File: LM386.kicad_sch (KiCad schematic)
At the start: 16 parts, among them J1 Conn_01x02_Pin, J2 Conn_01x02_Pin, U1 LM386, U2 LM386

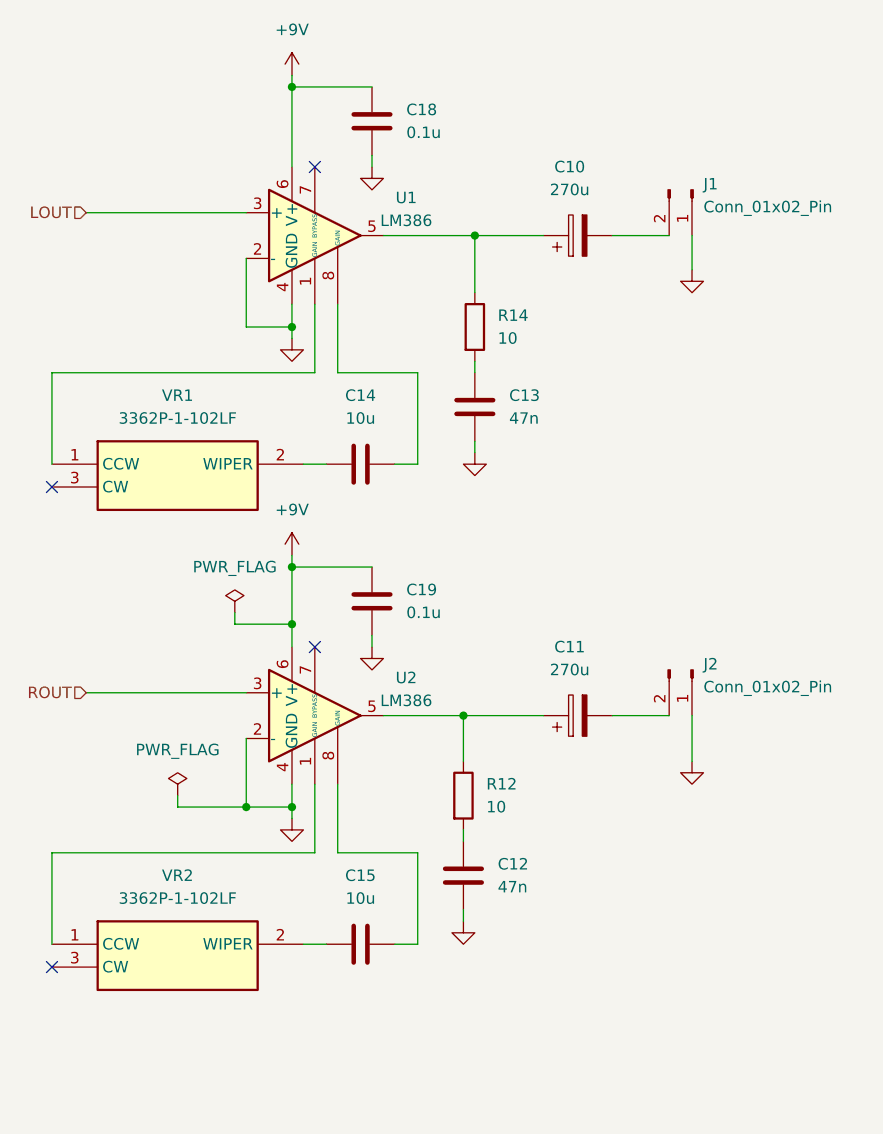
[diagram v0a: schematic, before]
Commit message: Complete layout
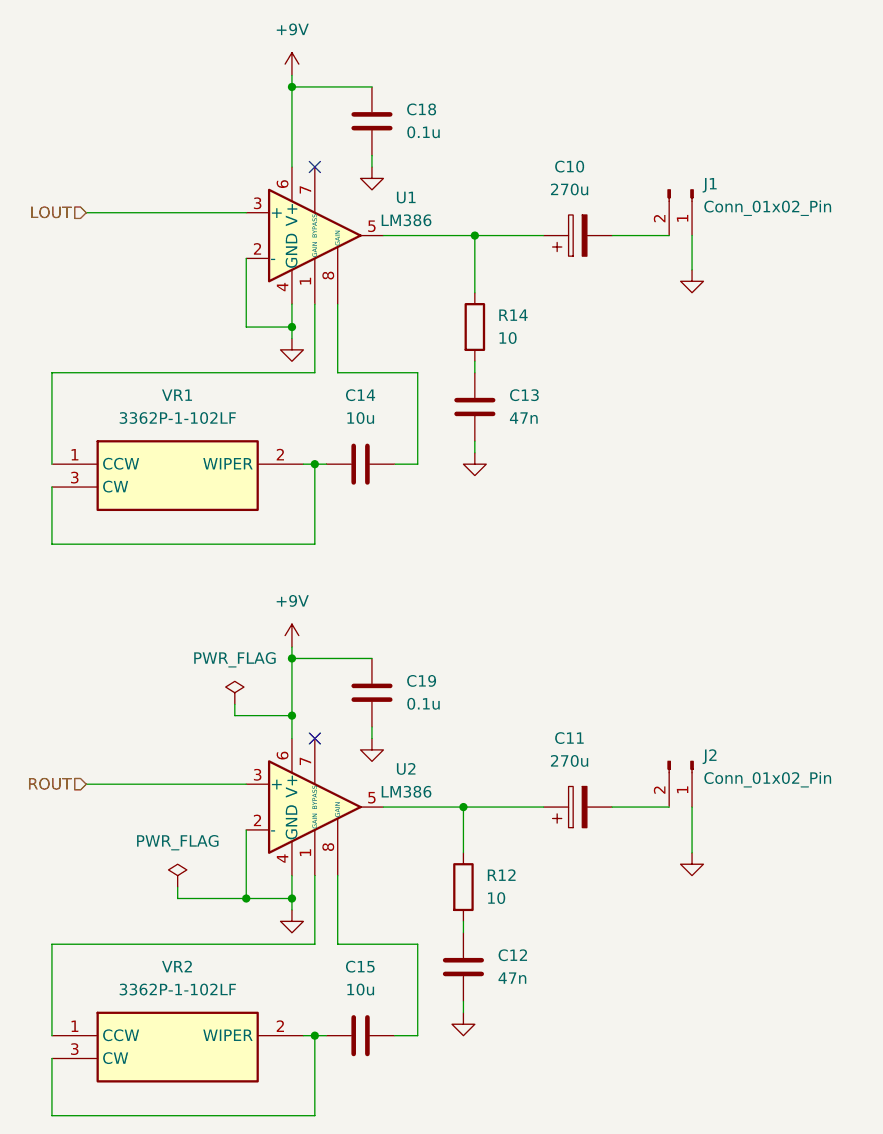
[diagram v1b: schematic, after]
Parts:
- R12, R14: footprint FM Radio:RESC1608X55N -> Resistor_SMD:R_0603_1608Metric
- VR1, VR2: footprint 3362P_1 -> FM Radio:3362P_1
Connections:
- net at C14.1, VR1.2 (WIPER): now also VR1.3 (CW)
- net at C15.1, VR2.2 (WIPER): now also VR2.3 (CW)
- no-connect marks 4 -> 2
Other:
- moved on the sheet: C11, C12, C15, C19, J2, R12, U2, VR2
